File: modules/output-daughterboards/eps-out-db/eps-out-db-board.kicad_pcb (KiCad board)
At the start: 4 copper layers, 43 x 20 mm, 7 parts, among them J1 EPS8 OUT FIELD, J10 TE 63951-1, J11 TE 63951-1, J12 TE 63951-1, J13 TE 63951-1, J14 TE 63951-1, J15 TE 63951-1

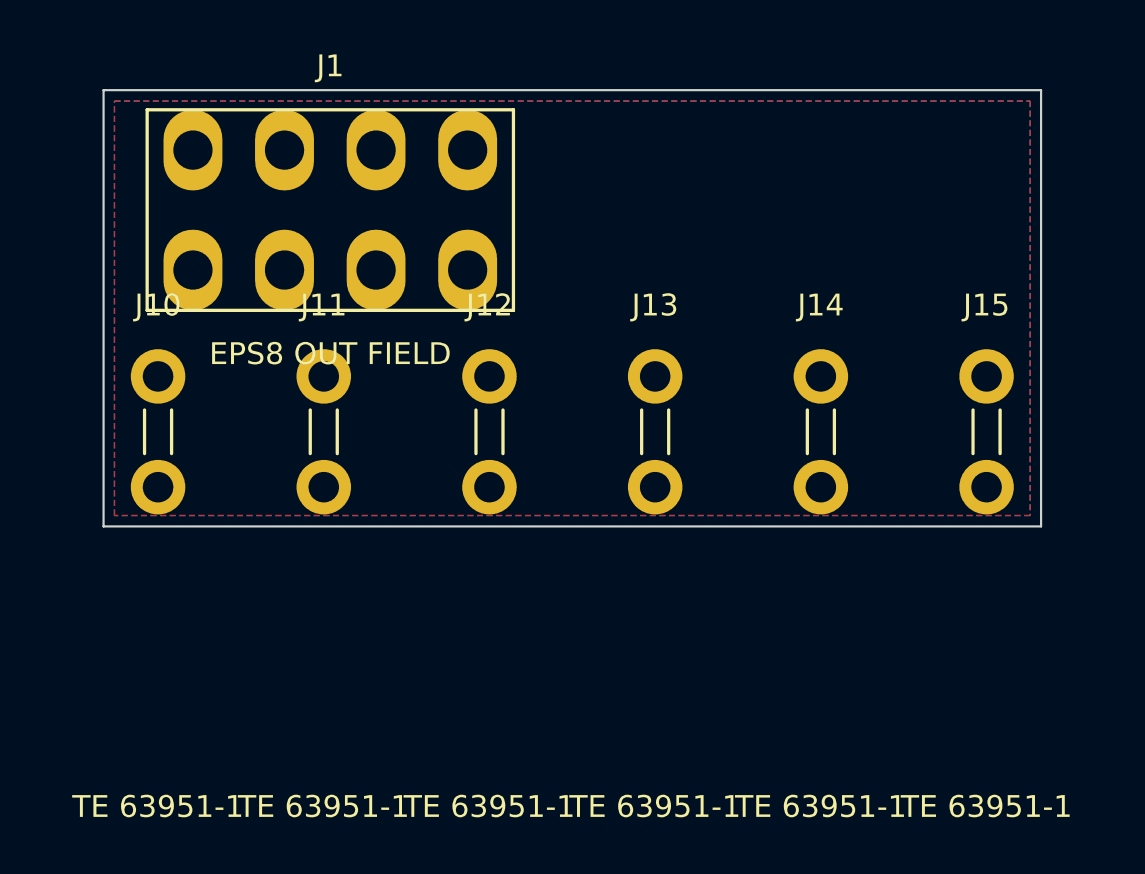
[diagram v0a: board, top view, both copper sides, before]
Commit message: WIP snapshot: iteration-5 boards regenerating + checker update in flight (durability)
Co-Authored-By: Claude Fable 5 <noreply@anthropic.com>
Claude-Session: https://claude.ai/code/session_01LvfqcnEeuin2oyJQw548EX
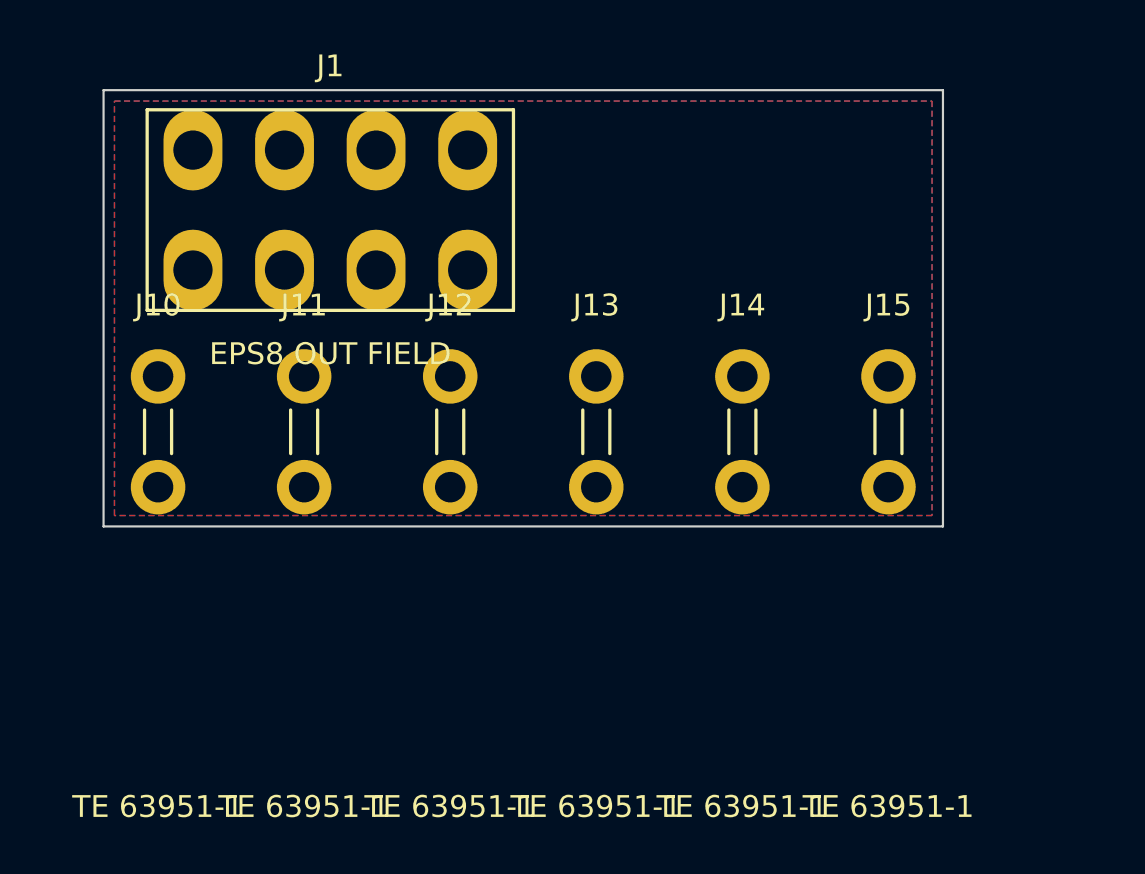
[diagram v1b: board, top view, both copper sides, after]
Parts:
- moved J15 4.50 mm to (36.0, 15.7)
- moved J14 3.60 mm to (29.3, 15.7)
- moved J13 2.70 mm to (22.6, 15.7)
- moved J12 1.80 mm to (15.9, 15.7)
- moved J11 0.90 mm to (9.20, 15.7)
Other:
- board size 43 x 20 mm -> 38.5 x 20 mm
